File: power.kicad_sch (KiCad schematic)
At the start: 54 parts, among them J8 USB_C_Receptacle_USB2.0_16P, Q2 Q_NMOS_GDS, SW2 SW_SPDT, U16 74LVC1G125, U2 BQ25895RTW, U4 LM1117DT-3.3, U5 MCP4017-xxxxLT, U7 LM3478MA

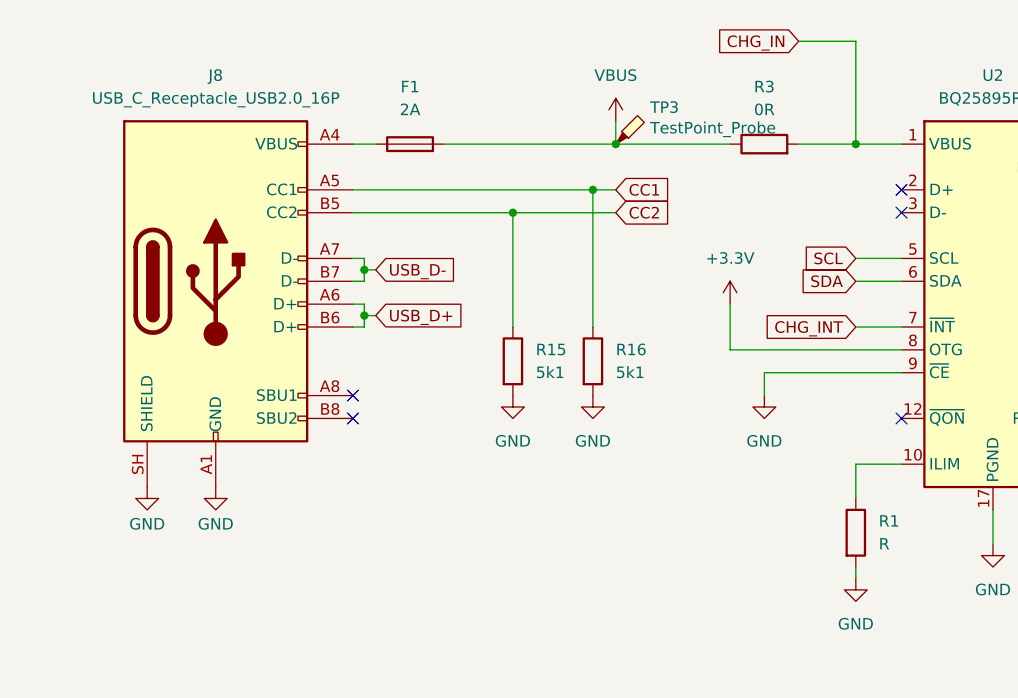
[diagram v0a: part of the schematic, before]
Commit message: Start routing
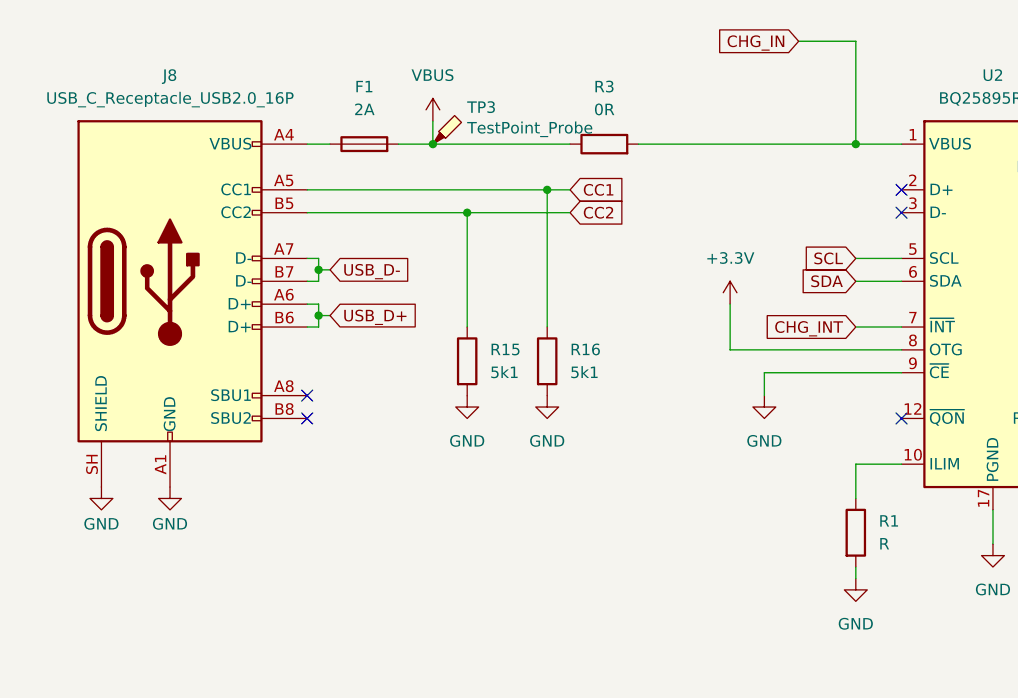
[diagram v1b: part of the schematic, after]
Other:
- moved on the sheet: F1, J8, R15, R16, R3, TP3
